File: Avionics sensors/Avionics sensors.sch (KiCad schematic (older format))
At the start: 9 parts, among them U1 STM32L151CCTx

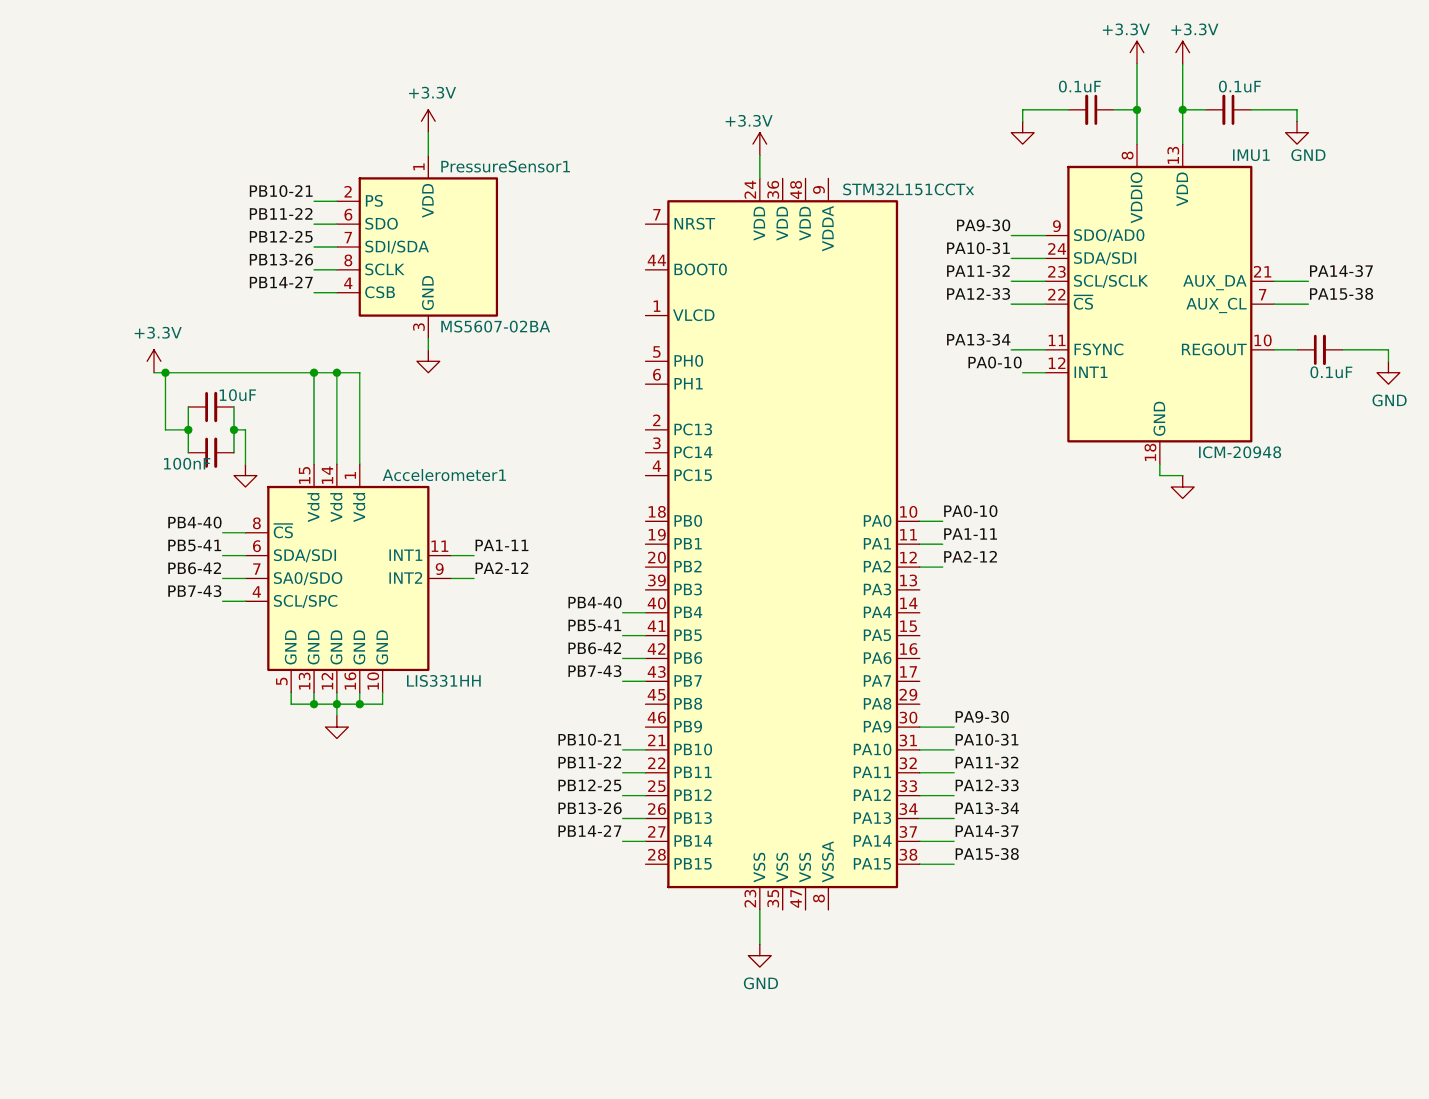
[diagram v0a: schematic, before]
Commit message: Add files via upload
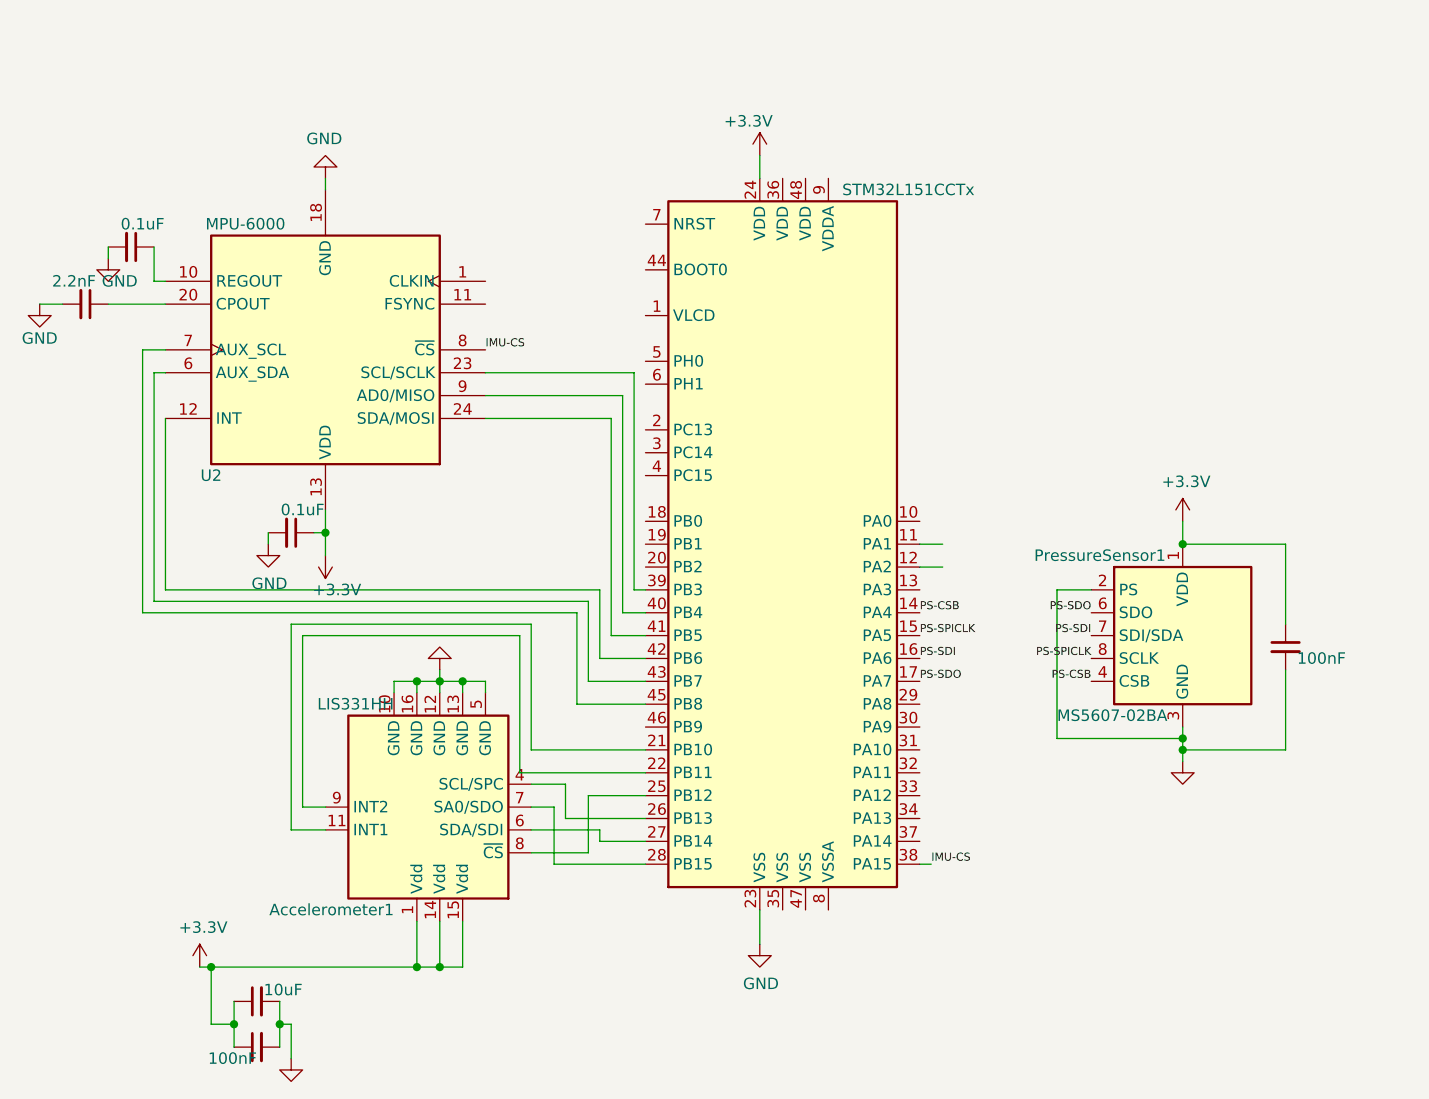
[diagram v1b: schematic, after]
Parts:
- removed C1, C2, C3: 0.1uF, symbol Device:C_Small
- removed IMU1: ICM-20948, Sensor_Motion:InvenSense_QFN-24_3x3mm_P0.4mm, symbol Sensor_Motion:ICM-20948
- added C-Ceramic2: 100nF, Capacitor_SMD:C_0805_2012Metric_Pad1.15x1.40mm_HandSolder, symbol Device:C_Small
- added C4, C5: 0.1uF, Capacitor_SMD:C_0805_2012Metric_Pad1.15x1.40mm_HandSolder, symbol Device:C_Small
- added C6: 2.2nF, Capacitor_SMD:C_0805_2012Metric_Pad1.15x1.40mm_HandSolder, symbol Device:C_Small
- added U2: MPU-6000, Sensor_Motion:InvenSense_QFN-24_4x4mm_P0.5mm, symbol Sensor_Motion:MPU-6000
- C-Aluminum1: footprint (none) -> Capacitor_SMD:CP_Elec_3x5.3
- C-Ceramic1: footprint (none) -> Capacitor_SMD:C_0805_2012Metric_Pad1.15x1.40mm_HandSolder
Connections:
- net +3V3: now also C-Ceramic2.1, C4.1, U2.13 (VDD)
- net GND: now also PressureSensor1.2 (PS), C-Ceramic2.2, C4.2, C5.2, C6.2, U2.18 (GND)
- net PS-CSB: now reaches U1.14 (PA4)
- net PS-CSB: now also PressureSensor1.4 (CSB), PressureSensor1.5 (CSB)
- net PS-SPICLK: now reaches U1.15 (PA5)
- net PS-SPICLK: now also PressureSensor1.8 (SCLK)
- net PS-SDI: now reaches U1.16 (PA6)
- net PS-SDI: now also PressureSensor1.7 (SDI/SDA)
- net PS-SDO: now reaches U1.17 (PA7)
- net PS-SDO: now also PressureSensor1.6 (SDO)
- net at U1.28 (PB15): now also Accelerometer1.7 (SA0/SDO)
- net at U1.39 (PB3): now also U2.23 (SCL/SCLK)
- net at U1.45 (PB8): now also U2.7 (AUX_SCL)
- net PA0-10: no longer names the net of U1.10 (PA0)
- net PA1-11: no longer names the net of U1.11 (PA1)
- net PA1-11: no longer Accelerometer1.11 (INT1)
- net PA10-31: no longer names the net of U1.31 (PA10)
- net PA11-32: no longer names the net of U1.32 (PA11)
- net PA12-33: no longer names the net of U1.33 (PA12)
- net PA13-34: no longer names the net of U1.34 (PA13)
- net PA14-37: no longer names the net of U1.37 (PA14)
- net PA15-38 renamed IMU-CS
- net IMU-CS: now also U2.8 (~CS)
- net PA2-12: no longer names the net of U1.12 (PA2)
- net PA2-12: no longer Accelerometer1.9 (INT2)
- net PA9-30: no longer names the net of U1.30 (PA9)
- net PB10-21: no longer names the net of U1.21 (PB10)
- net PB10-21: now also Accelerometer1.11 (INT1); no longer PressureSensor1.2 (PS)
- net PB11-22: no longer names the net of U1.22 (PB11)
- net PB11-22: now also Accelerometer1.9 (INT2); no longer PressureSensor1.6 (SDO)
- net PB12-25: no longer names the net of U1.25 (PB12)
- net PB12-25: now also Accelerometer1.8 (~CS); no longer PressureSensor1.7 (SDI/SDA)
- net PB13-26: no longer names the net of U1.26 (PB13)
- net PB13-26: now also Accelerometer1.4 (SCL/SPC); no longer PressureSensor1.8 (SCLK)
- removed net PB14-27: PressureSensor1.4 (CSB), PressureSensor1.5 (CSB), U1.27 (PB14)
- net PB4-40: no longer names the net of U1.40 (PB4)
- net PB4-40: now also U2.9 (AD0/MISO); no longer Accelerometer1.8 (~CS)
- net PB5-41: no longer names the net of Accelerometer1.6 (SDA/SDI)
- net PB5-41: now also U1.27 (PB14); no longer U1.41 (PB5)
- net PB6-42: no longer names the net of U1.42 (PB6)
- net PB6-42: now also U2.12 (INT); no longer Accelerometer1.7 (SA0/SDO)
- net PB7-43: no longer names the net of U1.43 (PB7)
- net PB7-43: now also U2.6 (AUX_SDA); no longer Accelerometer1.4 (SCL/SPC)
- new net: U1.41 (PB5), U2.24 (SDA/MOSI)
- new net: C5.1, U2.10 (REGOUT)
- new net: C6.1, U2.20 (CPOUT)
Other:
- moved on the sheet: Accelerometer1, PressureSensor1
